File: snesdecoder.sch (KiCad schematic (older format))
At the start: 12 parts, among them J1 SNES Controller Input, J2 Power, J3 12PAD, U1 74HC04, U2 74LS161, U3 TLC6C5912, U4 74LVC1G08

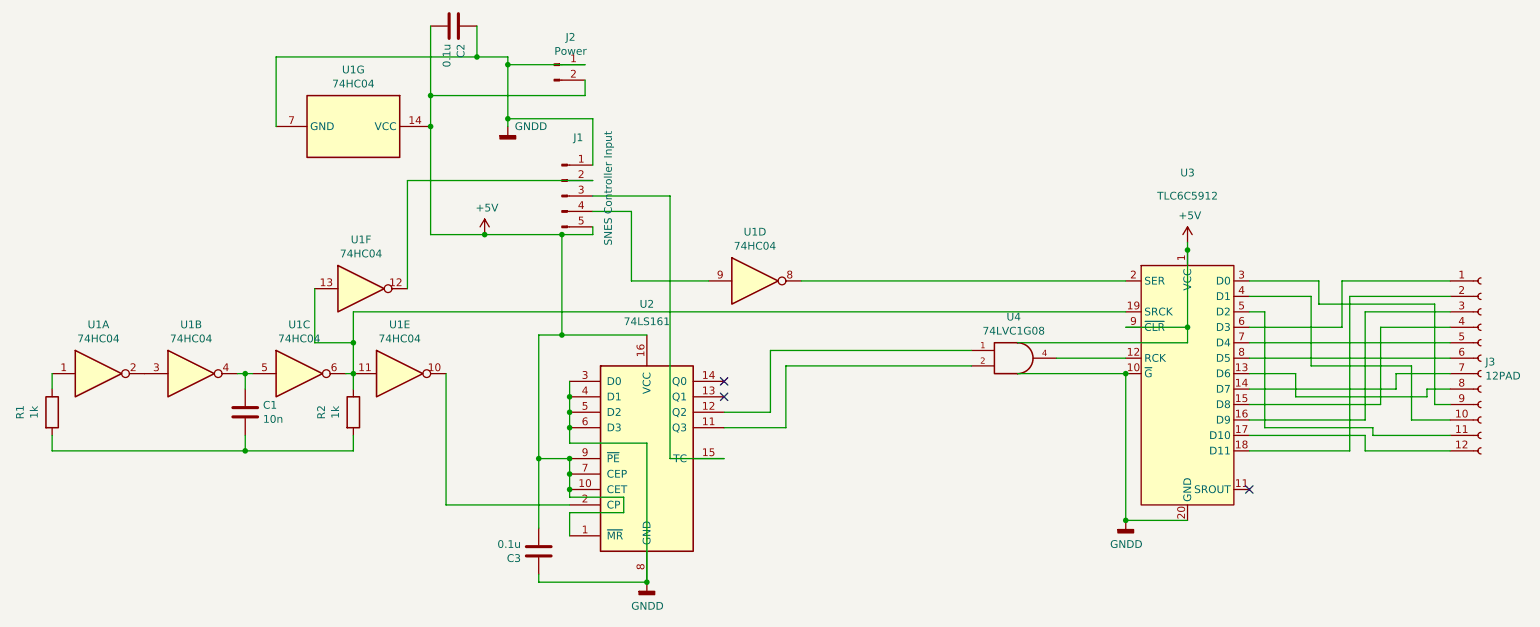
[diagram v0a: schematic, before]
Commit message: gerbers to v2
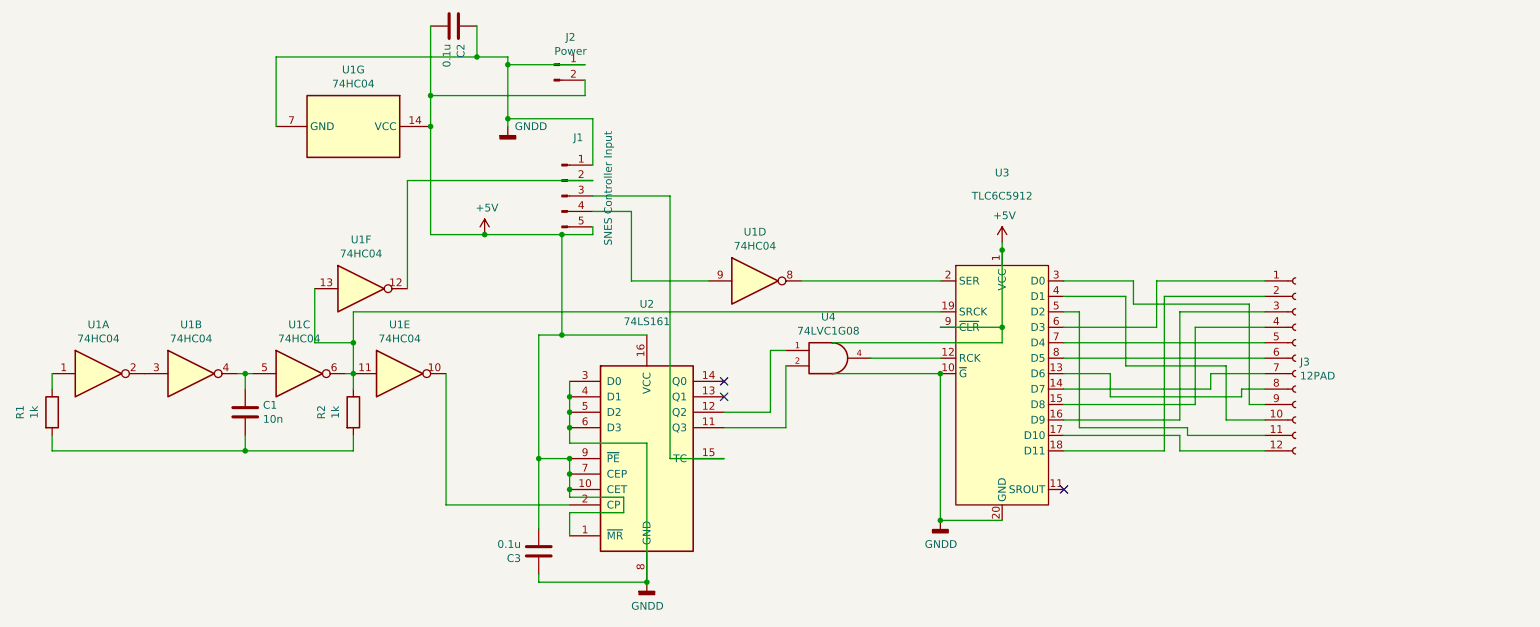
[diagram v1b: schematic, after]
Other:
- moved on the sheet: J3, U3, U4
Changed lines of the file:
@@
 L newchips:TLC6C5912 U3
 U 1 1 5FB36650
-P 8200 3350
-F 0 "U3" H 8200 4450 50  0000 C CNN
-F 1 "TLC6C5912" H 8200 4300 50  0000 C CNN
-F 2 "Package_SO:SOIC-20W_7.5x12.8mm_P1.27mm" H 8600 2650 50  0001 C CNN
-F 3 "" H 8600 2650 50  0001 C CNN
-	1    8200 3350
-	1    0    0    -1
-$EndComp
-Wire Wire Line
-	5700 2950 7800 2950
-Wire Wire Line
-	7350 3450 7800 3450
-Wire Wire Line
-	7800 3550 7800 4500
-Wire Wire Line
-	7800 4500 8200 4500
+P 7000 3350
+F 0 "U3" H 7000 4450 50  0000 C CNN
+F 1 "TLC6C5912" H 7000 4300 50  0000 C CNN
+F 2 "Package_SO:SOIC-20W_7.5x12.8mm_P1.27mm" H 7400 2650 50  0001 C CNN
+F 3 "" H 7400 2650 50  0001 C CNN
+	1    7000 3350
+	1    0    0    -1
+$EndComp
+Wire Wire Line
+	6150 3450 6600 3450
+Wire Wire Line
+	6600 3550 6600 4500
+Wire Wire Line
+	6600 4500 7000 4500
 $Comp
 L power:GNDD #PWR0101
 U 1 1 5FB3EC8C
-P 7800 4500
-F 0 "#PWR0101" H 7800 4250 50  0001 C CNN
-F 1 "GNDD" H 7804 4345 50  0000 C CNN
-F 2 "" H 7800 4500 50  0001 C CNN
-F 3 "" H 7800 4500 50  0001 C CNN
-	1    7800 4500
-	1    0    0    -1
-$EndComp
-Connection ~ 7800 4500
+P 6600 4500
+F 0 "#PWR0101" H 6600 4250 50  0001 C CNN
+F 1 "GNDD" H 6604 4345 50  0000 C CNN
+F 2 "" H 6600 4500 50  0001 C CNN
+F 3 "" H 6600 4500 50  0001 C CNN
+	1    6600 4500
+	1    0    0    -1
+$EndComp
+Connection ~ 6600 4500
 $Comp
 L power:+5V #PWR0102
 U 1 1 5FB41555
-P 8200 2700
-F 0 "#PWR0102" H 8200 2550 50  0001 C CNN
-F 1 "+5V" H 8215 2873 50  0000 C CNN
-F 2 "" H 8200 2700 50  0001 C CNN
-F 3 "" H 8200 2700 50  0001 C CNN
-	1    8200 2700
+P 7000 2700
+F 0 "#PWR0102" H 7000 2550 50  0001 C CNN
+F 1 "+5V" H 7015 2873 50  0000 C CNN
+F 2 "" H 7000 2700 50  0001 C CNN
+F 3 "" H 7000 2700 50  0001 C CNN
+	1    7000 2700
 	1    0    0    -1
 $EndComp
@@
 	4850 2400 4350 2400
 Wire Wire Line
-	7800 3250 8200 3250
-Wire Wire Line
-	8200 3250 8200 2750
-Wire Wire Line
-	8200 2750 8200 2700
-Connection ~ 8200 2750
+	6600 3250 7000 3250
+Wire Wire Line
+	7000 3250 7000 2750
+Wire Wire Line
+	7000 2750 7000 2700
+Connection ~ 7000 2750
 NoConn ~ 5200 3600
 NoConn ~ 5200 3700
-NoConn ~ 8600 4300
+NoConn ~ 7400 4300
 $Comp
 L 74xGxx:74LVC1G08 U4
 U 1 1 5FB0C867
-P 7100 3450
-F 0 "U4" H 7075 3717 50  0000 C CNN
-F 1 "74LVC1G08" H 7075 3626 50  0000 C CNN
-F 2 "Package_TO_SOT_SMD:SOT-353_SC-70-5_Handsoldering" H 7100 3450 50  0001 C CNN
-F 3 "http://www.ti.com/lit/sg/scyt129e/scyt129e.pdf" H 7100 3450 50  0001 C CNN
-	1    7100 3450
+P 5900 3450
+F 0 "U4" H 5875 3717 50  0000 C CNN
+F 1 "74LVC1G08" H 5875 3626 50  0000 C CNN
+F 2 "Package_TO_SOT_SMD:SOT-353_SC-70-5_Handsoldering" H 5900 3450 50  0001 C CNN
+F 3 "http://www.ti.com/lit/sg/scyt129e/scyt129e.pdf" H 5900 3450 50  0001 C CNN
+	1    5900 3450
 	1    0    0    -1
 $EndComp
@@
 	5500 3800 5500 3400
 Wire Wire Line
-	5500 3400 6800 3400
-Wire Wire Line
 	5600 3900 5600 3500
 Wire Wire Line
-	5600 3500 6800 3500
-Wire Wire Line
 	5200 3900 5600 3900
 Wire Wire Line
-	7100 3350 8200 3350
-Wire Wire Line
-	8200 3350 8200 3250
-Connection ~ 8200 3250
-Wire Wire Line
-	7100 3550 7800 3550
-Connection ~ 7800 3550
+	5900 3350 7000 3350
+Wire Wire Line
+	7000 3350 7000 3250
+Connection ~ 7000 3250
+Wire Wire Line
+	5900 3550 6600 3550
+Connection ~ 6600 3550
 $Comp
 L Device:R R2
@@
 Wire Wire Line
 	2800 3150 2800 3350
-Wire Wire Line
-	2800 3150 7800 3150
 Connection ~ 2800 3350
 $Comp
 L Connector:Conn_01x12_Female J3
 U 1 1 5FAF303D
-P 10100 3450
-F 0 "J3" H 10128 3426 50  0000 L CNN
-F 1 "12PAD" H 10128 3335 50  0000 L CNN
-F 2 "IO:12PAD" H 10100 3450 50  0001 C CNN
-F 3 "~" H 10100 3450 50  0001 C CNN
-	1    10100 3450
-	1    0    0    -1
-$EndComp
-Wire Wire Line
-	8600 4050 9250 4050
-Wire Wire Line
-	9250 4050 9250 3050
-Wire Wire Line
-	9250 3050 9900 3050
-Wire Wire Line
-	8600 3950 9350 3950
-Wire Wire Line
-	9350 3950 9350 4050
-Wire Wire Line
-	9350 4050 9900 4050
-Wire Wire Line
-	8600 3850 9350 3850
-Wire Wire Line
-	9350 3850 9350 3150
-Wire Wire Line
-	9350 3150 9900 3150
-Wire Wire Line
-	8600 3750 9450 3750
-Wire Wire Line
-	9450 3750 9450 3250
-Wire Wire Line
-	9450 3250 9900 3250
-Wire Wire Line
-	9550 3650 9550 3550
-Wire Wire Line
-	9550 3550 9900 3550
-Wire Wire Line
-	8600 3650 9550 3650
-Wire Wire Line
-	8600 3550 8900 3550
-Wire Wire Line
-	8900 3550 8900 3700
-Wire Wire Line
-	8900 3700 9750 3700
-Wire Wire Line
-	9750 3700 9750 3650
-Wire Wire Line
-	9750 3650 9900 3650
-Wire Wire Line
-	8600 3450 9900 3450
-Wire Wire Line
-	9900 3350 8600 3350
-Wire Wire Line
-	8600 3250 9200 3250
-Wire Wire Line
-	9200 3250 9200 2950
-Wire Wire Line
-	9200 2950 9900 2950
-Wire Wire Line
-	8600 3150 8700 3150
-Wire Wire Line
-	8700 3150 8700 3900
-Wire Wire Line
-	8700 3900 9400 3900
-Wire Wire Line
-	9400 3900 9400 3950
-Wire Wire Line
-	9400 3950 9900 3950
-Wire Wire Line
-	8600 3050 9000 3050
-Wire Wire Line
-	9000 3050 9000 3500
-Wire Wire Line
-	9000 3500 9650 3500
-Wire Wire Line
-	9650 3500 9650 3850
-Wire Wire Line
-	9650 3850 9900 3850
-Wire Wire Line
-	9900 3750 9800 3750
-Wire Wire Line
-	9800 3750 9800 3100
-Wire Wire Line
-	9800 3100 9050 3100
-Wire Wire Line
-	9050 3100 9050 2950
-Wire Wire Line
-	9050 2950 8600 2950
+P 8900 3450
+F 0 "J3" H 8928 3426 50  0000 L CNN
+F 1 "12PAD" H 8928 3335 50  0000 L CNN
+F 2 "IO:12PAD" H 8900 3450 50  0001 C CNN
+F 3 "~" H 8900 3450 50  0001 C CNN
+	1    8900 3450
+	1    0    0    -1
+$EndComp
+Wire Wire Line
+	7400 4050 8050 4050
+Wire Wire Line
+	8050 4050 8050 3050
+Wire Wire Line
+	8050 3050 8700 3050
+Wire Wire Line
+	7400 3950 8150 3950
+Wire Wire Line
+	8150 3950 8150 4050
+Wire Wire Line
+	8150 4050 8700 4050
+Wire Wire Line
+	7400 3850 8150 3850
+Wire Wire Line
+	8150 3850 8150 3150
+Wire Wire Line
+	8150 3150 8700 3150
+Wire Wire Line
+	7400 3750 8250 3750
+Wire Wire Line
+	8250 3750 8250 3250
+Wire Wire Line
+	8250 3250 8700 3250
+Wire Wire Line
+	8350 3650 8350 3550
+Wire Wire Line
+	8350 3550 8700 3550
+Wire Wire Line
+	7400 3650 8350 3650
+Wire Wire Line
+	7400 3550 7700 3550
+Wire Wire Line
+	7700 3550 7700 3700
+Wire Wire Line
+	7700 3700 8550 3700
+Wire Wire Line
+	8550 3700 8550 3650
+Wire Wire Line
+	8550 3650 8700 3650
+Wire Wire Line
+	7400 3450 8700 3450
+Wire Wire Line
+	8700 3350 7400 3350
+Wire Wire Line
+	7400 3250 8000 3250
+Wire Wire Line
+	8000 3250 8000 2950
+Wire Wire Line
+	8000 2950 8700 2950
+Wire Wire Line
+	7400 3150 7500 3150
+Wire Wire Line
+	7500 3150 7500 3900
+Wire Wire Line
+	7500 3900 8200 3900
+Wire Wire Line
+	8200 3900 8200 3950
+Wire Wire Line
+	8200 3950 8700 3950
+Wire Wire Line
+	7400 3050 7800 3050
+Wire Wire Line
+	7800 3050 7800 3500
+Wire Wire Line
+	7800 3500 8450 3500
+Wire Wire Line
+	8450 3500 8450 3850
+Wire Wire Line
+	8450 3850 8700 3850
+Wire Wire Line
+	8700 3750 8600 3750
+Wire Wire Line
+	8600 3750 8600 3100
+Wire Wire Line
+	8600 3100 7850 3100
+Wire Wire Line
+	7850 3100 7850 2950
+Wire Wire Line
+	7850 2950 7400 2950
+Wire Wire Line
+	5700 2950 6600 2950
+Wire Wire Line
+	6600 3150 2800 3150
+Wire Wire Line
+	5500 3400 5600 3400
 $EndSCHEMATC

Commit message: fix sch
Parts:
- U1: footprint Package_SO:SOIC-14_3.9x8.7mm_P1.27mm -> Package_SO:TSSOP-14_4.4x5mm_P0.65mm
- U2: footprint Package_SO:SOIC-16_3.9x9.9mm_P1.27mm -> Package_SO:TSSOP-16_4.4x5mm_P0.65mm
- U3: footprint Package_SO:SOIC-20W_7.5x12.8mm_P1.27mm -> Package_SO:TSSOP-20_4.4x6.5mm_P0.65mm
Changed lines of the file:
@@
 F 0 "U2" H 4700 5100 50  0000 C CNN
 F 1 "74LS161" H 4700 4987 50  0000 C CNN
-F 2 "Package_SO:SOIC-16_3.9x9.9mm_P1.27mm" H 4700 4100 50  0001 C CNN
+F 2 "Package_SO:TSSOP-16_4.4x5mm_P0.65mm" H 4700 4100 50  0001 C CNN
 F 3 "http://www.ti.com/lit/gpn/sn74LS161" H 4700 4100 50  0001 C CNN
 	1    4700 4100
@@
 F 0 "U3" H 7000 4450 50  0000 C CNN
 F 1 "TLC6C5912" H 7000 4300 50  0000 C CNN
-F 2 "Package_SO:SOIC-20W_7.5x12.8mm_P1.27mm" H 7400 2650 50  0001 C CNN
+F 2 "Package_SO:TSSOP-20_4.4x6.5mm_P0.65mm" H 7400 2650 50  0001 C CNN
 F 3 "" H 7400 2650 50  0001 C CNN
 	1    7000 3350
@@
 F 0 "U1" H 1150 3867 50  0000 C CNN
 F 1 "74HC04" H 1150 3776 50  0000 C CNN
-F 2 "Package_SO:SOIC-14_3.9x8.7mm_P1.27mm" H 1150 3550 50  0001 C CNN
+F 2 "Package_SO:TSSOP-14_4.4x5mm_P0.65mm" H 1150 3550 50  0001 C CNN
 F 3 "https://assets.nexperia.com/documents/data-sheet/74HC_HCT04.pdf" H 1150 3550 50  0001 C CNN
 	1    1150 3550
@@
 F 0 "U1" H 1750 3867 50  0000 C CNN
 F 1 "74HC04" H 1750 3776 50  0000 C CNN
-F 2 "Package_SO:SOIC-14_3.9x8.7mm_P1.27mm" H 1750 3550 50  0001 C CNN
+F 2 "Package_SO:TSSOP-14_4.4x5mm_P0.65mm" H 1750 3550 50  0001 C CNN
 F 3 "https://assets.nexperia.com/documents/data-sheet/74HC_HCT04.pdf" H 1750 3550 50  0001 C CNN
 	2    1750 3550
@@
 F 0 "U1" H 2450 3867 50  0000 C CNN
 F 1 "74HC04" H 2450 3776 50  0000 C CNN
-F 2 "Package_SO:SOIC-14_3.9x8.7mm_P1.27mm" H 2450 3550 50  0001 C CNN
+F 2 "Package_SO:TSSOP-14_4.4x5mm_P0.65mm" H 2450 3550 50  0001 C CNN
 F 3 "https://assets.nexperia.com/documents/data-sheet/74HC_HCT04.pdf" H 2450 3550 50  0001 C CNN
 	3    2450 3550
@@
 F 0 "U1" V 2433 1950 50  0000 C CNN
 F 1 "74HC04" V 2524 1950 50  0000 C CNN
-F 2 "Package_SO:SOIC-14_3.9x8.7mm_P1.27mm" H 2800 1950 50  0001 C CNN
+F 2 "Package_SO:TSSOP-14_4.4x5mm_P0.65mm" H 2800 1950 50  0001 C CNN
 F 3 "https://assets.nexperia.com/documents/data-sheet/74HC_HCT04.pdf" H 2800 1950 50  0001 C CNN
 	7    2800 1950
@@
 F 0 "U1" H 5400 3267 50  0000 C CNN
 F 1 "74HC04" H 5400 3176 50  0000 C CNN
-F 2 "Package_SO:SOIC-14_3.9x8.7mm_P1.27mm" H 5400 2950 50  0001 C CNN
+F 2 "Package_SO:TSSOP-14_4.4x5mm_P0.65mm" H 5400 2950 50  0001 C CNN
 F 3 "https://assets.nexperia.com/documents/data-sheet/74HC_HCT04.pdf" H 5400 2950 50  0001 C CNN
 	4    5400 2950
@@
 F 0 "U1" H 3100 3867 50  0000 C CNN
 F 1 "74HC04" H 3100 3776 50  0000 C CNN
-F 2 "Package_SO:SOIC-14_3.9x8.7mm_P1.27mm" H 3100 3550 50  0001 C CNN
+F 2 "Package_SO:TSSOP-14_4.4x5mm_P0.65mm" H 3100 3550 50  0001 C CNN
 F 3 "https://assets.nexperia.com/documents/data-sheet/74HC_HCT04.pdf" H 3100 3550 50  0001 C CNN
 	5    3100 3550
@@
 F 0 "U1" H 2850 3317 50  0000 C CNN
 F 1 "74HC04" H 2850 3226 50  0000 C CNN
-F 2 "Package_SO:SOIC-14_3.9x8.7mm_P1.27mm" H 2850 3000 50  0001 C CNN
+F 2 "Package_SO:TSSOP-14_4.4x5mm_P0.65mm" H 2850 3000 50  0001 C CNN
 F 3 "https://assets.nexperia.com/documents/data-sheet/74HC_HCT04.pdf" H 2850 3000 50  0001 C CNN
 	6    2850 3000
